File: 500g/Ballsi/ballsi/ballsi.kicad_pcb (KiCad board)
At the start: 2 copper layers, 90 x 59 mm, 28 parts, among them K1 G6DN-1A-SL DC12, SW1 1101M2S3CQE2

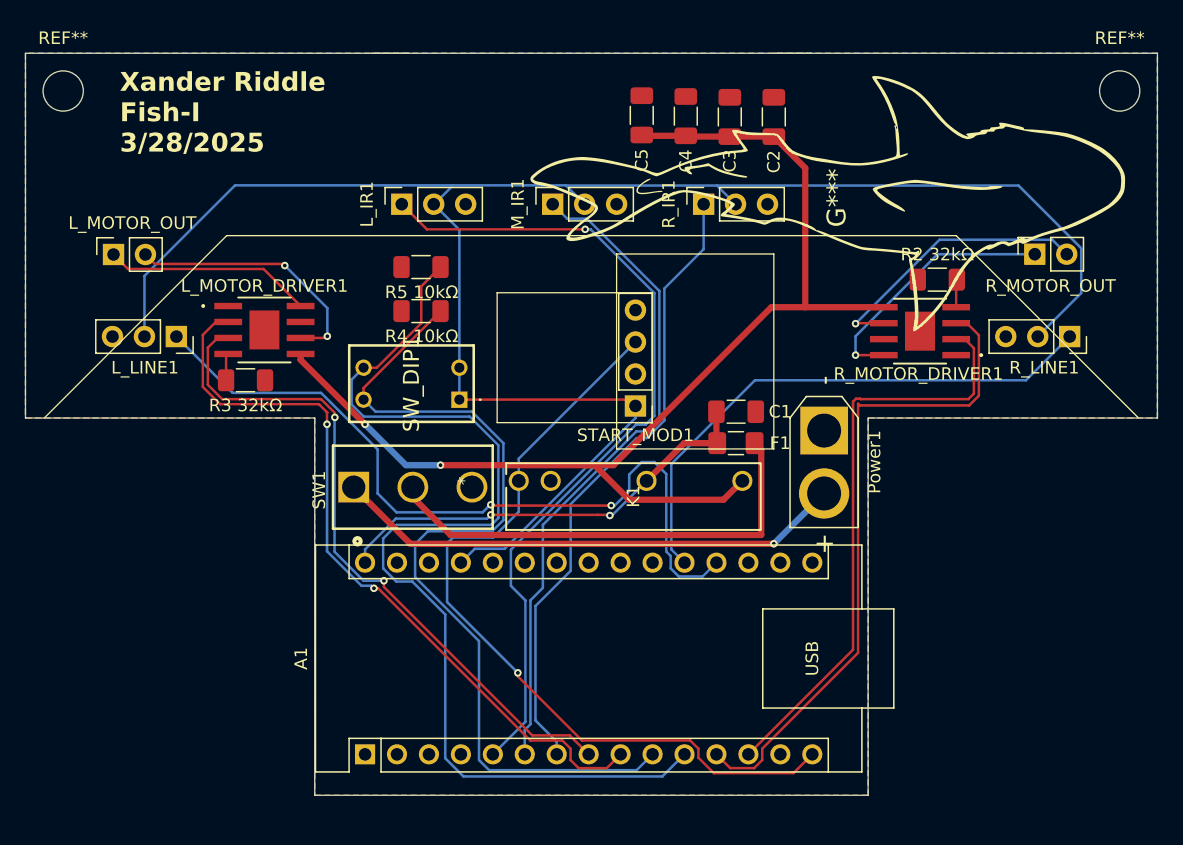
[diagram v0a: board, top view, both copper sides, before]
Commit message: finished v2s
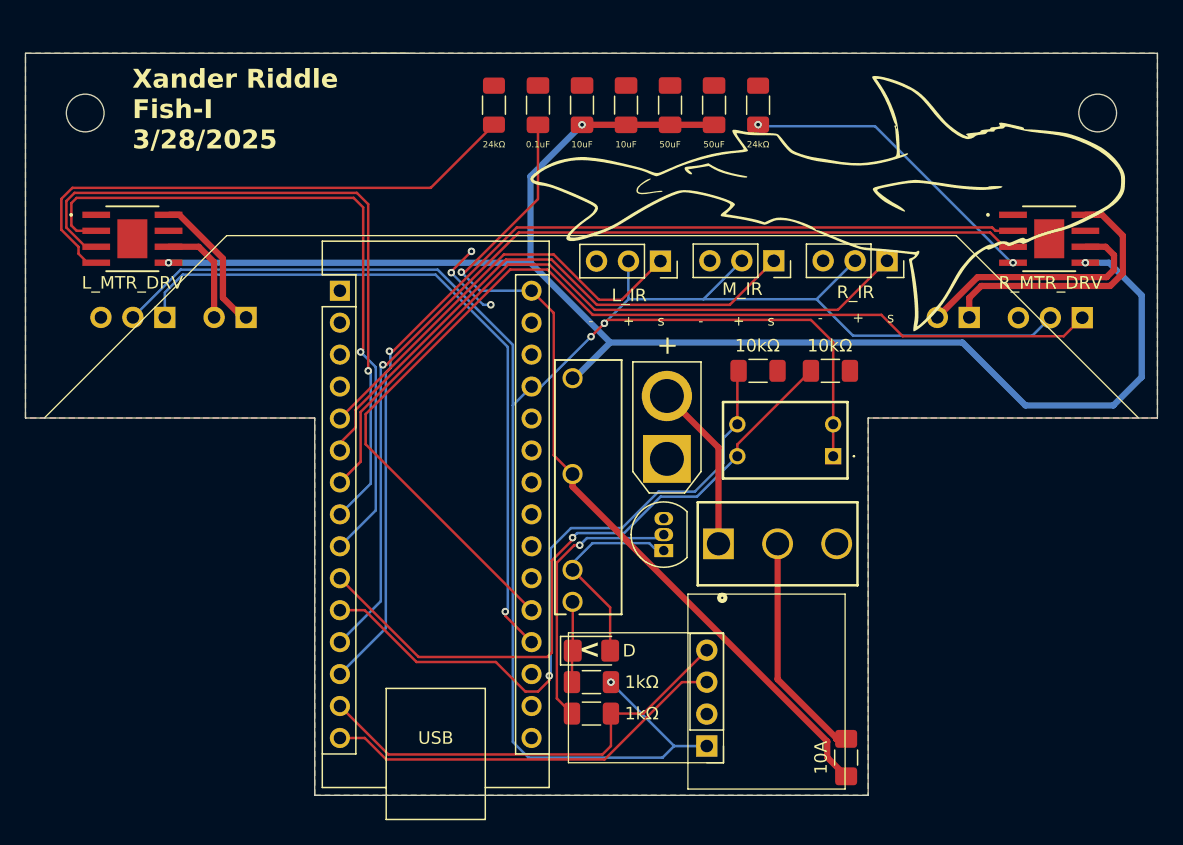
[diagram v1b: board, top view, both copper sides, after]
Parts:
- removed the REF** at (153.5, 53.0)
- removed the REF** at (237.5, 53.0)
- added 1kΩ: R, Resistor_SMD:R_1206_3216Metric_Pad1.30x1.75mm_HandSolder, F.Cu at (195.5, 100.0)
- added 1kΩ: R, Resistor_SMD:R_1206_3216Metric_Pad1.30x1.75mm_HandSolder, F.Cu at (195.5, 102.5)
- added D: D, Diode_SMD:D_1206_3216Metric_Pad1.42x1.75mm_HandSolder, F.Cu at (195.5, 97.5)
- added Q1: BC549, Package_TO_SOT_THT:TO-92_Inline, F.Cu at (201.2, 89.5)
- added REF**: MountingHole_3mm, MountingHole:MountingHole_3mm, F.Cu at (155.2, 54.8)
- added REF**: MountingHole_3mm, MountingHole:MountingHole_3mm, F.Cu at (235.8, 54.8)
- 10kΩ: renamed from R4 10kΩ
- 10kΩ: renamed from R5 10kΩ
- 24kΩ: renamed from R3 32kΩ; value 32kΩ -> 24kΩ
- 24kΩ: renamed from R2 32kΩ; value 32kΩ -> 24kΩ
- 50uF: renamed from C4; value 10uF -> 50uF
- 50uF: renamed from C2; value 10uF -> 50uF
- moved A1 36.9 mm to (175.5, 68.9), turned to 0 degrees
- moved 10kΩ 32.9 mm to (214.5, 75.2), turned to 180 degrees
- moved SW_DIP1 30.1 mm to (214.7, 82.0)
- moved 24kΩ 29.5 mm to (187.8, 54.1), turned to 90 degrees
- moved SW1 29.3 mm to (210.3, 89.0)
- moved 0.1uF 29.0 mm to (191.2, 54.1), turned to 90 degrees
- moved 10kΩ 28.0 mm to (208.8, 75.2), turned to 180 degrees
- moved START_MOD1 27.6 mm to (204.7, 105.1)
- moved 10A 26.5 mm to (215.8, 106.0), turned to 90 degrees
- moved L_IR 21.1 mm to (201.0, 66.5), turned to -90 degrees
- moved 24kΩ 19.9 mm to (208.8, 54.1), turned to 90 degrees
- moved M_IR 18.1 mm to (210.0, 66.5), turned to -90 degrees
- moved R_IR 15.3 mm to (219.0, 66.5), turned to -90 degrees
- moved L_MTR_DRV 12.8 mm to (159.0, 64.8)
- moved Power1 12.7 mm to (201.5, 82.2), turned to 90 degrees
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- renumbered C1 to 0.1uF, F1 to 10A, C3 to 10uF, C5 to 10uF, L_MOTOR_OUT to J1, R_MOTOR_OUT to J2, L_IR1 to L_IR, L_MOTOR_DRIVER1 to L_MTR_DRV, M_IR1 to M_IR, R_IR1 to R_IR, R_MOTOR_DRIVER1 to R_MTR_DRV
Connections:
- A1 pad 14: unconnected-(A1-D11-Pad14) -> Kill_Switch
- K1 pad 1: START_MOD -> Net-(D1-K)
- K1 pad 2: GND -> Net-(D1-A)
- START_MOD1 pad 4: unconnected-(START_MOD1-Pin_4-Pad4) -> Kill_Switch
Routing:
- net R_LINE: track 44.2 -> 85.6 mm
- net Net-(L_MOTOR_DRIVER1-ILIM): track 2.17 -> 43.5 mm
- net Kill_Switch: track 0.00 -> 35.7 mm
- net +12V: track 35.1 -> 69.6 mm, vias 2 -> 1
- net R_IN2: track 47.7 -> 81.1 mm, vias 0 -> 1
- net L_IR: track 66.4 -> 33.7 mm, vias 1 -> 0
- net START_MOD: track 64.6 -> 32.4 mm, vias 1 -> 0
- net DIP2: track 83.7 -> 54.6 mm, vias 0 -> 1
- net MOTOR_PWR: track 94.9 -> 122.5 mm, vias 2 -> 3
- net Net-(Power1-Pin_2): track 40.9 -> 13.4 mm, vias 1 -> 0
- net +5V: track 150.1 -> 177.1 mm, vias 0 -> 3
- net R_IN1: track 52.8 -> 78.4 mm, vias 0 -> 1
- net Net-(R_MOTOR_DRIVER1-ILIM): track 2.21 -> 24.8 mm, vias 0 -> 2
- net Net-(Q1-B): track 0.00 -> 21.9 mm, vias 0 -> 1
- net Net-(F1-Pad2): track 37.3 -> 18.2 mm
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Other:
- board text added: "+"
- board text added: "-"
- board text added: "<"
- board text added: "L_Line"
- board text added: "L_MTR"
- board text added: "R_Line"
- board text added: "R_MTR"
- board text added: "s"
